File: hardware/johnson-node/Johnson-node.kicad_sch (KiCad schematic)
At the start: 86 parts, among them IC1 ADC124S051CIMM_NOPB, IC2 ADC124S051CIMM_NOPB, J1 Conn_01x02, J10 Conn_01x03, J11 Conn_01x03, J13 BSEL, J14 RST, J15 SO4B-XASK-1, J16 Conn_01x02, J17 Conn_01x14, J2 Conn_01x03, J3 Conn_01x03, J4 Conn_01x03, J5 Conn_01x03, J6 Conn_01x03, J7 Conn_01x03, J8 Conn_01x03, J9 Conn_01x03, U1 ESP32-S3-WROOM-1U-N4R2, U2 LMR50410Y3FQDBVRQ1, U3 LMR50410Y5FQDBVRQ1, U4 ISO1042BQDWVQ1, U5 MAX3390EEUD_T, U6 MAX3390EEUD_T

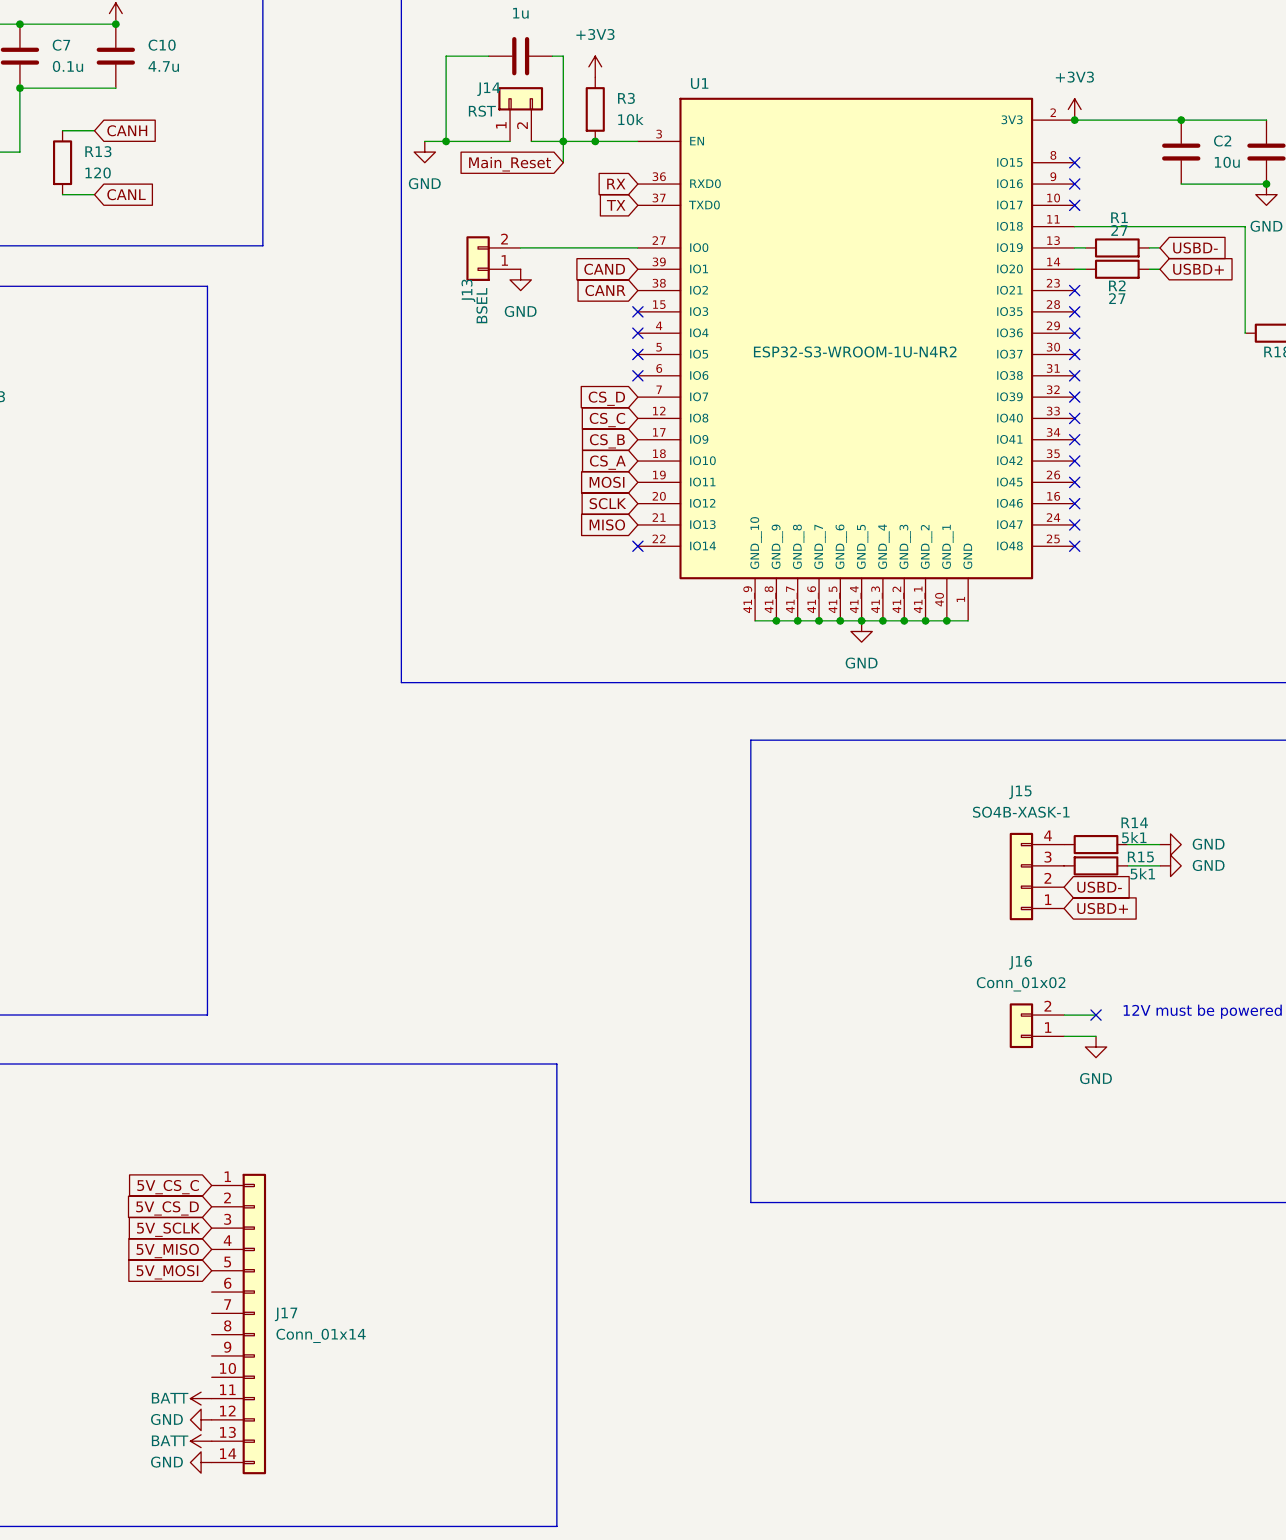
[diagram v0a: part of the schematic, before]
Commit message: add onboard reg
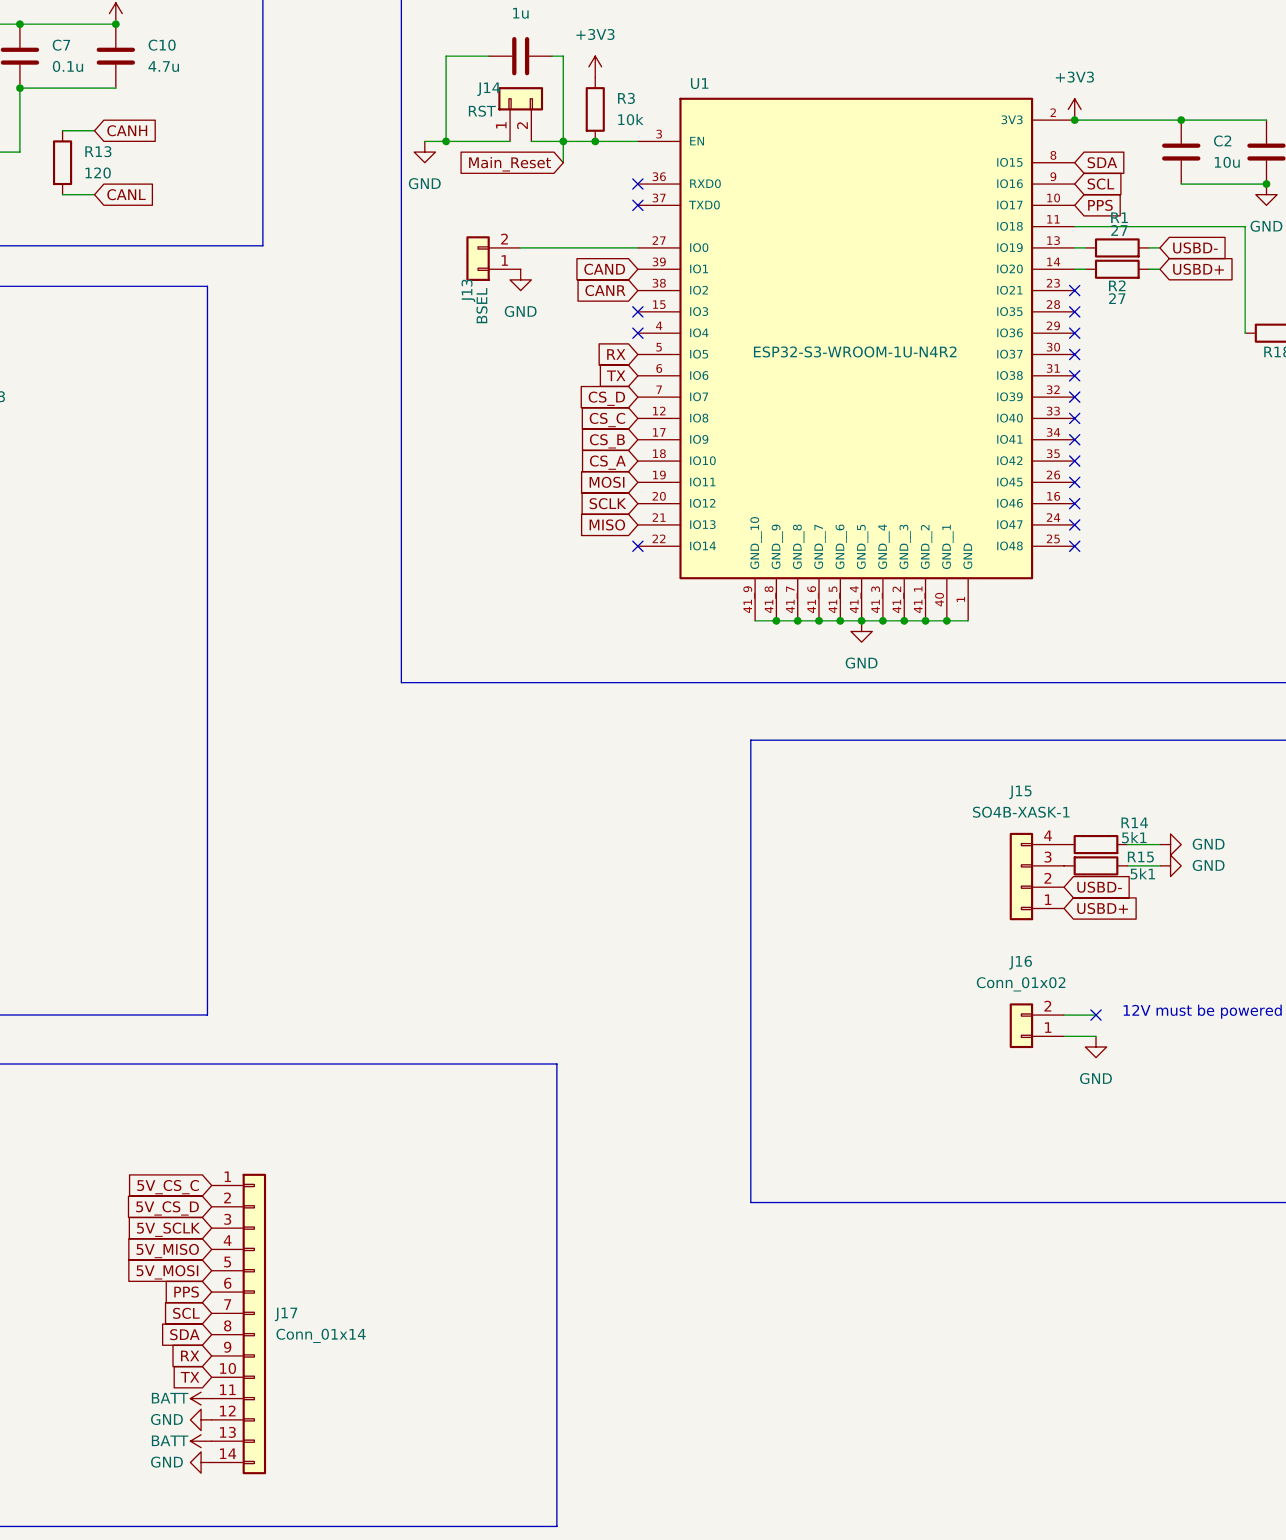
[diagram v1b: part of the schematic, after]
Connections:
- net RX: now also J17.9 (Pin_9), U1.5 (IO5); no longer U1.36 (RXD0)
- net TX: now also J17.10 (Pin_10), U1.6 (IO6); no longer U1.37 (TXD0)
- net PPS: now reaches J17.6 (Pin_6)
- net PPS: now also U1.10 (IO17)
- net SCL: now reaches J17.7 (Pin_7)
- net SCL: now also U1.9 (IO16)
- net SDA: now reaches J17.8 (Pin_8)
- net SDA: now also U1.8 (IO15)
- no-connect marks 24 -> 21
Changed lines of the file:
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@@
 	)
 	(no_connect
-		(at 295.91 73.66)
+		(at 347.98 86.36)
 	)
 	(no_connect
-		(at 347.98 86.36)
+		(at 295.91 53.34)
 	)
 	(no_connect
@@
 	)
 	(no_connect
-		(at 347.98 50.8)
-	)
-	(no_connect
 		(at 152.4 119.38)
 	)
@@
 	)
 	(no_connect
-		(at 295.91 71.12)
-	)
-	(no_connect
 		(at 347.98 93.98)
 	)
 	(no_connect
-		(at 347.98 53.34)
+		(at 295.91 50.8)
 	)
 	(no_connect
@@
 	)
 	(no_connect
-		(at 347.98 48.26)
-	)
-	(no_connect
 		(at 347.98 88.9)
 	)
@@
 		)
 	)
-	(global_label "TX"
+	(global_label "SCL"
 		(shape input)
-		(at 295.91 53.34 180)
+		(at 347.98 50.8 0)
 		(fields_autoplaced yes)
 		(effects
@@
 				(size 1.27 1.27)
 			)
-			(justify right)
+			(justify left)
 		)
 		(property "Intersheetrefs" "${INTERSHEET_REFS}"
-			(at 290.7477 53.34 0)
+			(at 354.4728 50.8 0)
 			(hide yes)
 			(show_name no)
@@
 					(size 1.27 1.27)
 				)
-				(justify right)
+				(justify left)
 			)
 		)
@@
 		)
 	)
+	(global_label "TX"
+		(shape input)
+		(at 295.91 73.66 180)
+		(fields_autoplaced yes)
+		(effects
+			(font
+				(size 1.27 1.27)
+			)
+			(justify right)
+		)
+		(property "Intersheetrefs" "${INTERSHEET_REFS}"
+			(at 290.7477 73.66 0)
+			(hide yes)
+			(show_name no)
+			(do_not_autoplace no)
+			(effects
+				(font
+					(size 1.27 1.27)
+				)
+				(justify right)
+			)
+		)
+	)
 	(global_label "5V_CS_C"
 		(shape input)
@@
 		)
 	)
-	(global_label "RX"
+	(global_label "PPS"
 		(shape input)
-		(at 295.91 50.8 180)
+		(at 347.98 53.34 0)
 		(fields_autoplaced yes)
 		(effects
@@
 				(size 1.27 1.27)
 			)
-			(justify right)
+			(justify left)
 		)
 		(property "Intersheetrefs" "${INTERSHEET_REFS}"
-			(at 290.4453 50.8 0)
+			(at 354.7147 53.34 0)
 			(hide yes)
 			(show_name no)
@@
 					(size 1.27 1.27)
 				)
-				(justify right)
+				(justify left)
 			)
 		)
@@
 		)
 	)
+	(global_label "PPS"
+		(shape input)
+		(at 245.11 182.88 180)
+		(fields_autoplaced yes)
+		(effects
+			(font
+				(size 1.27 1.27)
+			)
+			(justify right)
+		)
+		(property "Intersheetrefs" "${INTERSHEET_REFS}"
+			(at 238.3753 182.88 0)
+			(hide yes)
+			(show_name no)
+			(do_not_autoplace no)
+			(effects
+				(font
+					(size 1.27 1.27)
+				)
+				(justify right)
+			)
+		)
+	)
 	(global_label "SGF_P"
 		(shape input)
@@
 		)
 	)
+	(global_label "RX"
+		(shape input)
+		(at 295.91 71.12 180)
+		(fields_autoplaced yes)
+		(effects
+			(font
+				(size 1.27 1.27)
+			)
+			(justify right)
+		)
+		(property "Intersheetrefs" "${INTERSHEET_REFS}"
+			(at 290.4453 71.12 0)
+			(hide yes)
+			(show_name no)
+			(do_not_autoplace no)
+			(effects
+				(font
+					(size 1.27 1.27)
+				)
+				(justify right)
+			)
+		)
+	)
 	(global_label "SGB"
 		(shape input)
@@
 		)
 	)
+	(global_label "RX"
+		(shape input)
+		(at 245.11 190.5 180)
+		(fields_autoplaced yes)
+		(effects
+			(font
+				(size 1.27 1.27)
+			)
+			(justify right)
+		)
+		(property "Intersheetrefs" "${INTERSHEET_REFS}"
+			(at 239.6453 190.5 0)
+			(hide yes)
+			(show_name no)
+			(do_not_autoplace no)
+			(effects
+				(font
+					(size 1.27 1.27)
+				)
+				(justify right)
+			)
+		)
+	)
 	(global_label "SGG"
 		(shape input)
@@
 		)
 	)
+	(global_label "TX"
+		(shape input)
+		(at 245.11 193.04 180)
+		(fields_autoplaced yes)
+		(effects
+			(font
+				(size 1.27 1.27)
+			)
+			(justify right)
+		)
+		(property "Intersheetrefs" "${INTERSHEET_REFS}"
+			(at 239.9477 193.04 0)
+			(hide yes)
+			(show_name no)
+			(do_not_autoplace no)
+			(effects
+				(font
+					(size 1.27 1.27)
+				)
+				(justify right)
+			)
+		)
+	)
 	(global_label "USBD+"
 		(shape input)
@@
 		)
 	)
+	(global_label "SDA"
+		(shape input)
+		(at 245.11 187.96 180)
+		(fields_autoplaced yes)
+		(effects
+			(font
+				(size 1.27 1.27)
+			)
+			(justify right)
+		)
+		(property "Intersheetrefs" "${INTERSHEET_REFS}"
+			(at 238.5567 187.96 0)
+			(hide yes)
+			(show_name no)
+			(do_not_autoplace no)
+			(effects
+				(font
+					(size 1.27 1.27)
+				)
+				(justify right)
+			)
+		)
+	)
 	(global_label "SGG_P"
 		(shape input)
@@
 		)
 	)
+	(global_label "SCL"
+		(shape input)
+		(at 245.11 185.42 180)
+		(fields_autoplaced yes)
+		(effects
+			(font
+				(size 1.27 1.27)
+			)
+			(justify right)
+		)
+		(property "Intersheetrefs" "${INTERSHEET_REFS}"
+			(at 238.6172 185.42 0)
+			(hide yes)
+			(show_name no)
+			(do_not_autoplace no)
+			(effects
+				(font
+					(size 1.27 1.27)
+				)
+				(justify right)
+			)
+		)
+	)
 	(global_label "5V_CS_B"
 		(shape input)
@@
 			)
 		)
+	)
+	(global_label "SDA"
+		(shape input)
+		(at 347.98 48.26 0)
+		(fields_autoplaced yes)
+		(effects
+			(font
+				(size 1.27 1.27)
+			)
+			(justify left)
+		)
+		(property "Intersheetrefs" "${INTERSHEET_REFS}"
+			(at 354.5333 48.26 0)
+			(hide yes)
+			(show_name no)
+			(do_not_autoplace no)
+			(effects
+				(font
+					(size 1.27 1.27)
+				)
+				(justify left)
+			)
+		)

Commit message: 3d models
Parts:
- L1, L2: footprint CustomFootprints:Shielded_Inductor_SMD_7265 -> CustomFootprints:WE-TPC_4828
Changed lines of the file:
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@@
 			)
 		)
-		(property "Footprint" "CustomFootprints:Shielded_Inductor_SMD_7265"
+		(property "Footprint" "CustomFootprints:WE-TPC_4828"
 			(at 64.77 78.74 0)
 			(hide yes)
@@
 			)
 		)
-		(property "Footprint" "CustomFootprints:Shielded_Inductor_SMD_7265"
+		(property "Footprint" "CustomFootprints:WE-TPC_4828"
 			(at 68.58 118.11 0)
 			(hide yes)
